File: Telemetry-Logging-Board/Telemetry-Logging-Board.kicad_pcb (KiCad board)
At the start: 4 copper layers, 43.8 x 66.3 mm, 57 parts, among them J1 Raspberry_Pi_4, J2 Heltec Thingimagiger, J3 Main, J6 AUX_CAN, J8 USB_C_Receptacle_USB2.0_16P, J9 21992304, U1 PCF8523T, U10 FT234XD, U2 AP63205WU, U3 MIC5504-3.3YM5, U4 MCP2518FD-xQBB, U5 ISO1044BD, U6 MCP2518FD-xQBB, U7 ISO1044BD, U8 MCP2518FD-xQBB, U9 ISO1044BD, Y1 32.768 kHz Quartz Crystal, Y2 ECS-200-12-33Q-JES-TR, Y3 ECS-200-12-33Q-JES-TR, Y4 ECS-200-12-33Q-JES-TR

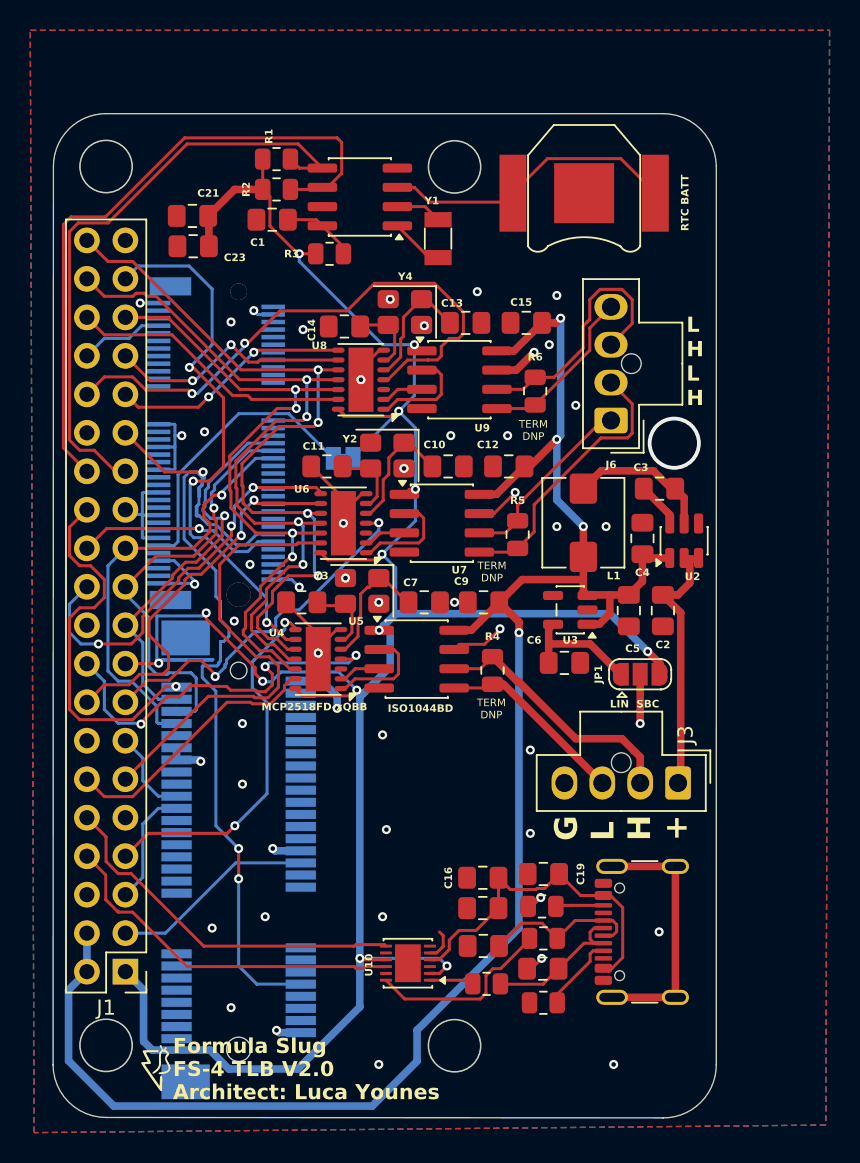
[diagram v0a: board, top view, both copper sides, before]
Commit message: complete routing less power
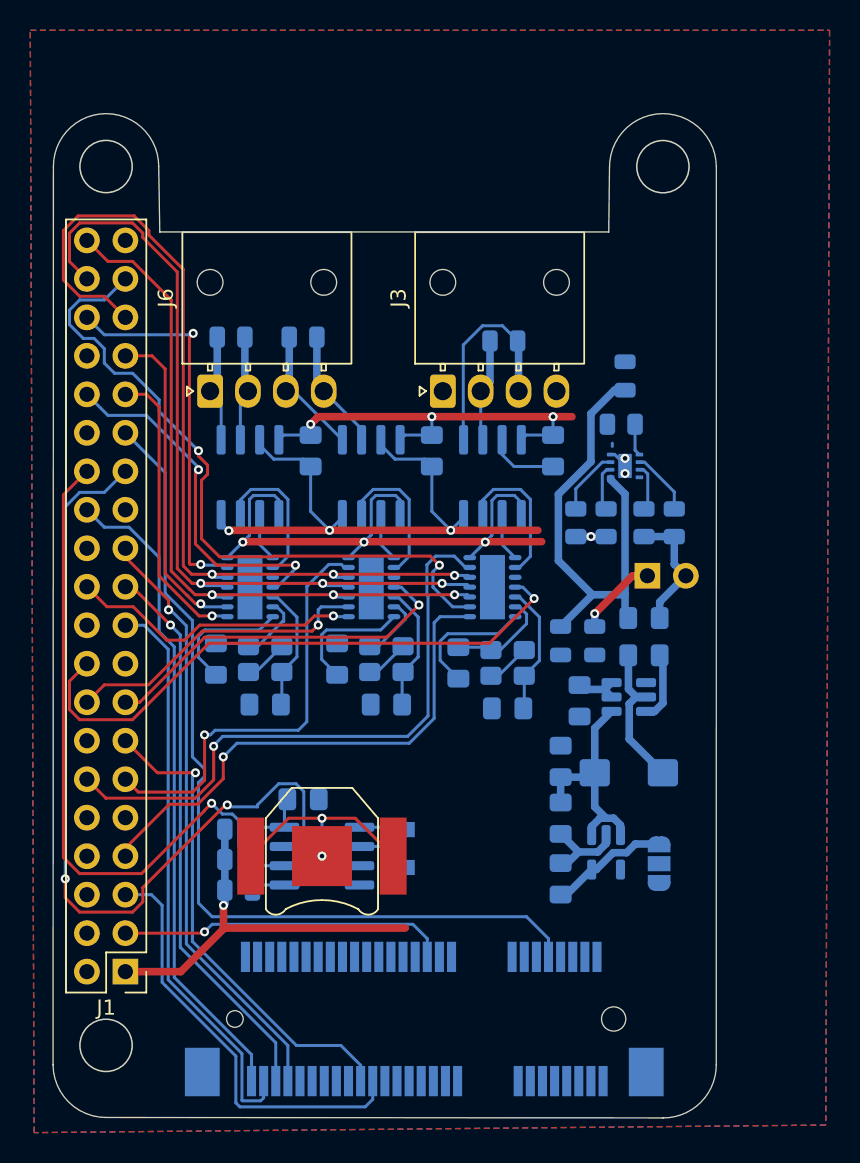
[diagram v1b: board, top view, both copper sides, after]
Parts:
- removed C17, C18: 47pF, Capacitor_SMD:C_0805_2012Metric_Pad1.18x1.45mm_HandSolder
- removed C19, C21, C23: 100nF, Capacitor_SMD:C_0805_2012Metric_Pad1.18x1.45mm_HandSolder
- removed C22: 4.7uF, Capacitor_SMD:C_0805_2012Metric_Pad1.18x1.45mm_HandSolder
- removed G***: , formula_slug_footprint_library:FORMULA SLUG TITLE
- removed J8: USB_C_Receptacle_USB2.0_16P, Connector_USB:USB_C_Receptacle_GCT_USB4105-xx-A_16P_TopMnt_Horizontal
- removed J9: 21992304, formula_slug_footprint_library:CONN-SMD_AS0BC21-S48BE-7H
- removed JP2: SolderJumper_2_Open, Jumper:SolderJumper-2_P1.3mm_Bridged_Pad1.0x1.5mm
- added BT2: 6S Ni-Mih, Connector_PinHeader_2.54mm:PinHeader_1x02_P2.54mm_Vertical, B.Cu at (160.7, 58.2)
- added D1: D_Shockley, Diode_SMD:D_0805_2012Metric, B.Cu at (159.2, 45.1)
- added D2: D_Shockley, Diode_SMD:D_0805_2012Metric, B.Cu at (157.2, 62.5)
- added D3: D_Shockley, Diode_SMD:D_0805_2012Metric, B.Cu at (155.0, 62.5)
- added R11: 10k, Resistor_SMD:R_0805_2012Metric, B.Cu at (156.0, 54.8)
- C1, C10, C11, C12, C13, C14, C15, C2, C3, C4, C5, C6, C7, C8, C9, JP1, L1, R1, R2, R3, R4, R5, R6, U1, U2, U3, U4, U5, U6, U7, U8, U9, Y1, Y2, Y3, Y4: moved to B.Cu
- C16: value 10nF -> 1uF; moved to B.Cu
- J3, J6: footprint Connector_Molex:Molex_Nano-Fit_105309-xx04_1x04_P2.50mm_Vertical -> Connector_Molex:Molex_Nano-Fit_105313-xx04_1x04_P2.50mm_Horizontal
- R10: value 5.1kΩ -> 18k; moved to B.Cu
- R7: value 5.1kΩ -> 604R; moved to B.Cu
- R8: value 27Ω -> 4.6k; moved to B.Cu
- R9: value 27Ω -> V_set; moved to B.Cu
- U10: value FT234XD -> BQ25172DSGR; footprint Package_DFN_QFN:WDFN-12-1EP_3x3mm_P0.45mm_EP1.7x2.5mm -> formula_slug_footprint_library:IC_BQ25172DSGR; moved to B.Cu
- moved R1 48.3 mm to (133.8, 79.0)
- moved BT1 47.0 mm to (139.2, 76.8)
- moved R2 44.3 mm to (133.8, 77.0)
- moved U1 43.6 mm to (139.2, 76.8)
- moved Y1 40.3 mm to (144.5, 76.2), turned to -90 degrees
- moved R3 38.4 mm to (133.8, 75.0)
- moved C1 38.3 mm to (138.0, 73.0), turned to 0 degrees
- moved U10 35.8 mm to (159.2, 51.0), turned to 0 degrees
- moved R9 34.3 mm to (159.0, 48.2)
- moved R8 32.2 mm to (160.5, 54.8), turned to -90 degrees
- moved R7 31.9 mm to (158.0, 54.8), turned to -90 degrees
- moved J3 30.2 mm to (147.2, 46.1), turned to 90 degrees
- moved C13 28.5 mm to (135.5, 66.8), turned to 180 degrees
- moved R10 26.8 mm to (162.5, 54.8), turned to -90 degrees
- moved J6 26.5 mm to (131.9, 46.1), turned to 90 degrees
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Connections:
- C16 pad 2: Net-(U10-VCC) -> +12V
- C2 pad 2: +12V -> Net-(D2-K)
- J1 pad 10: /PI_RX -> unconnected-(J1-GPIO15/UART_RXD-Pad10)
- J1 pad 24: /RF_SPI_~{CS} -> /CHRG
- J1 pad 8: /PI_TX -> unconnected-(J1-GPIO14/UART_TXD-Pad8)
- J3 pad 1: +12V -> /12V_RAW
- J6 pad 1: /Can interface and transiever1/CAN_H -> /Can interface and transiever2/CAN_L
- J6 pad 2: /Can interface and transiever1/CAN_L -> /Can interface and transiever2/CAN_H
- J6 pad 3: /Can interface and transiever2/CAN_H -> /Can interface and transiever1/CAN_L
- J6 pad 4: /Can interface and transiever2/CAN_L -> /Can interface and transiever1/CAN_H
- R10 pad 1: Net-(J8-CC2) -> Net-(U10-TMR)
- R7 pad 1: Net-(J8-CC1) -> Net-(U10-ISET)
- R8 pad 1: Net-(C18-Pad1) -> Net-(U10-VSET)
- R8 pad 2: Net-(U10-USBDM) -> GND
- R9 pad 1: Net-(C17-Pad1) -> /CHRG
- R9 pad 2: Net-(U10-USBDP) -> /SBC_3v3
- U10 pad 1: Net-(U10-USBDM) -> +12V
- U10 pad 2: /SBC_3v3 -> Net-(U10-ISET)
- U10 pad 3: unconnected-(U10-3V3OUT-Pad3) -> Net-(U10-TS)
- U10 pad 4: Net-(U10-VCC) -> GND
- U10 pad 5: GND -> /CHRG
- U10 pad 6: unconnected-(U10-CBUS0-Pad6) -> Net-(U10-TMR)
- U10 pad 7: /PI_RX -> Net-(U10-VSET)
- U10 pad 8: unconnected-(U10-~{RTS}/D2-Pad8) -> Net-(BT2-+)
- U10 pad 9: /SBC_3v3 -> GND
- U2 pad 2: +12V -> Net-(D2-K)
- U2 pad 3: +12V -> Net-(D2-K)
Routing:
- net /SBC_3v3: track 172.5 -> 69.0 mm, vias 13 -> 4
- net +5V: track 120.2 -> 42.7 mm, vias 4 -> 3
- net GND: track 65.3 -> 103.0 mm, vias 44 -> 7
- net /RF_HT_WAKE: track 5.77 -> 32.3 mm, vias 0 -> 1
- net /PI_RX: track 24.3 -> 0.00 mm
- net /PI_TX: track 23.8 -> 0.00 mm
- net Net-(U10-VCC): track 23.0 -> 0.00 mm
- net /CAN0_~{CS}: track 17.7 -> 40.0 mm, vias 0 -> 1
- net /RF_HT_BUSY: track 7.80 -> 28.3 mm
- net /SDA_I2C1: track 40.4 -> 60.9 mm, vias 0 -> 2
- net Net-(JP2-B): track 19.0 -> 0.00 mm
- net /RF_SPI_~{CS}1: track 24.8 -> 43.2 mm, vias 1 -> 0
- net unconnected-(J8-SHIELD-PadS1): track 17.0 -> 0.00 mm
- net +3V3: track 16.2 -> 0.00 mm, vias 7 -> 0
- net +12V: track 17.1 -> 31.5 mm
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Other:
- outline, holes or cut-outs redrawn
- board text removed: "G L H +"
- board text removed: "L H L H"
- board text removed: "LIN SBC"
- board text removed: "RTC BATT"
- board text removed: "TERM DNP"
